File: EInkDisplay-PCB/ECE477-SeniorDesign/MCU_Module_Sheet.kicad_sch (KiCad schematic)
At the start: 20 parts, among them SW1 SW_Push_Dual_x2, U3 STM32L496ZGTxP

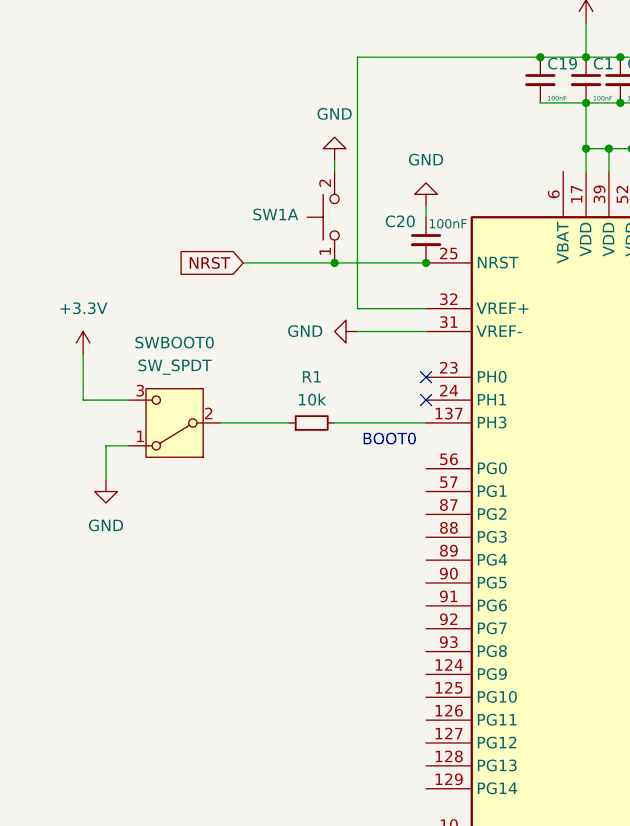
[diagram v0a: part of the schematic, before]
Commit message: Changes
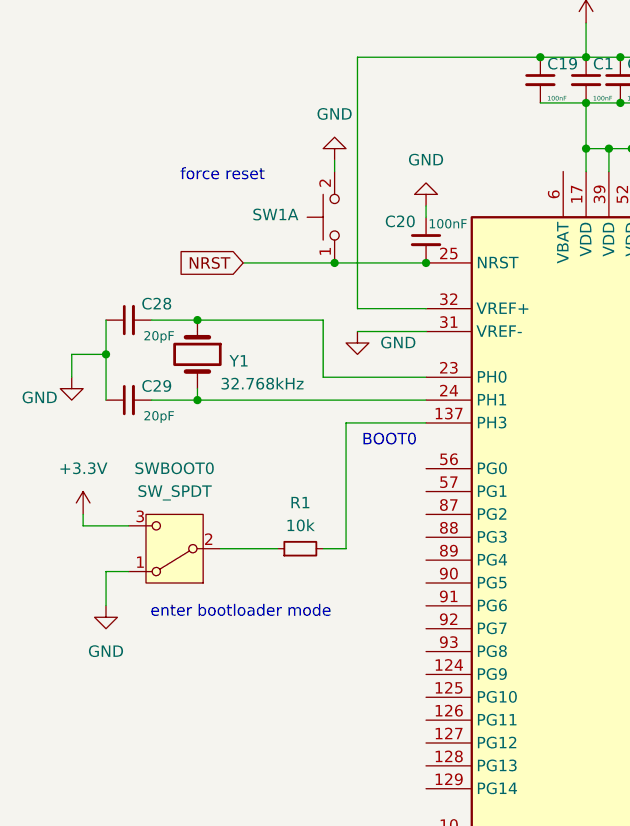
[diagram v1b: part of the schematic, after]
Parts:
- added C28, C29: 20pF, symbol Device:C_Small
- added Y1: 32.768kHz, symbol Device:Crystal
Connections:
- net GND: now also C28.1, C29.1
- net at U3.23 (PH0): now also C28.2, Y1.1
- net at U3.24 (PH1): now also C29.2, Y1.2
- no-connect marks 5 -> 3
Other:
- note added: "enter bootloader mode"
- note added: "force reset"
- moved on the sheet: R1, SWBOOT0

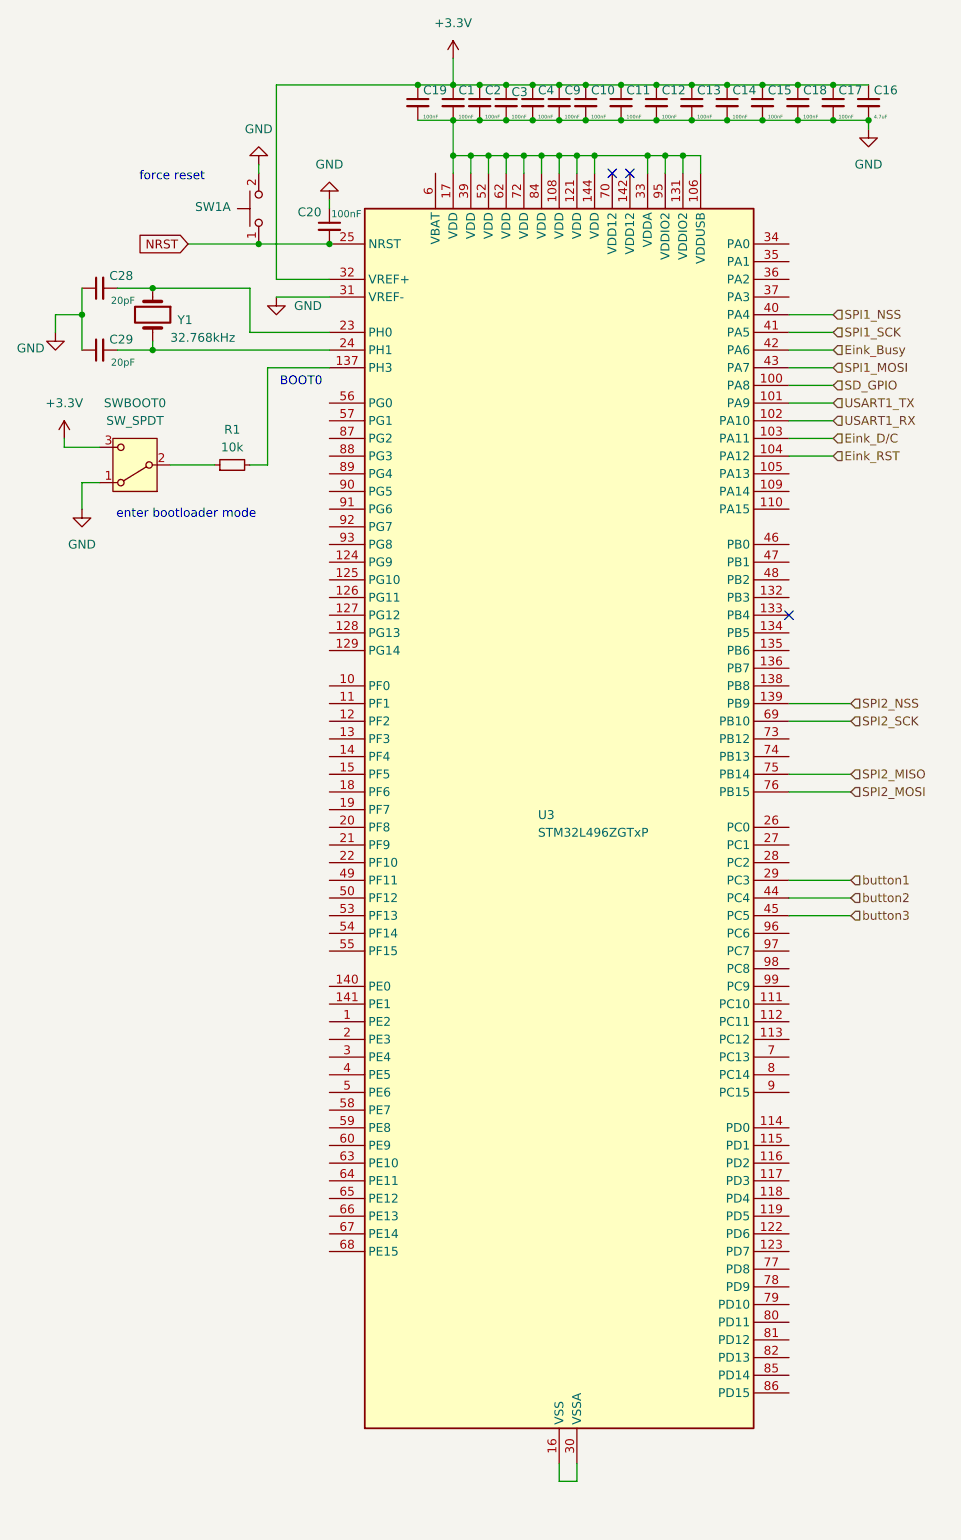
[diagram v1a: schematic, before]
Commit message: push
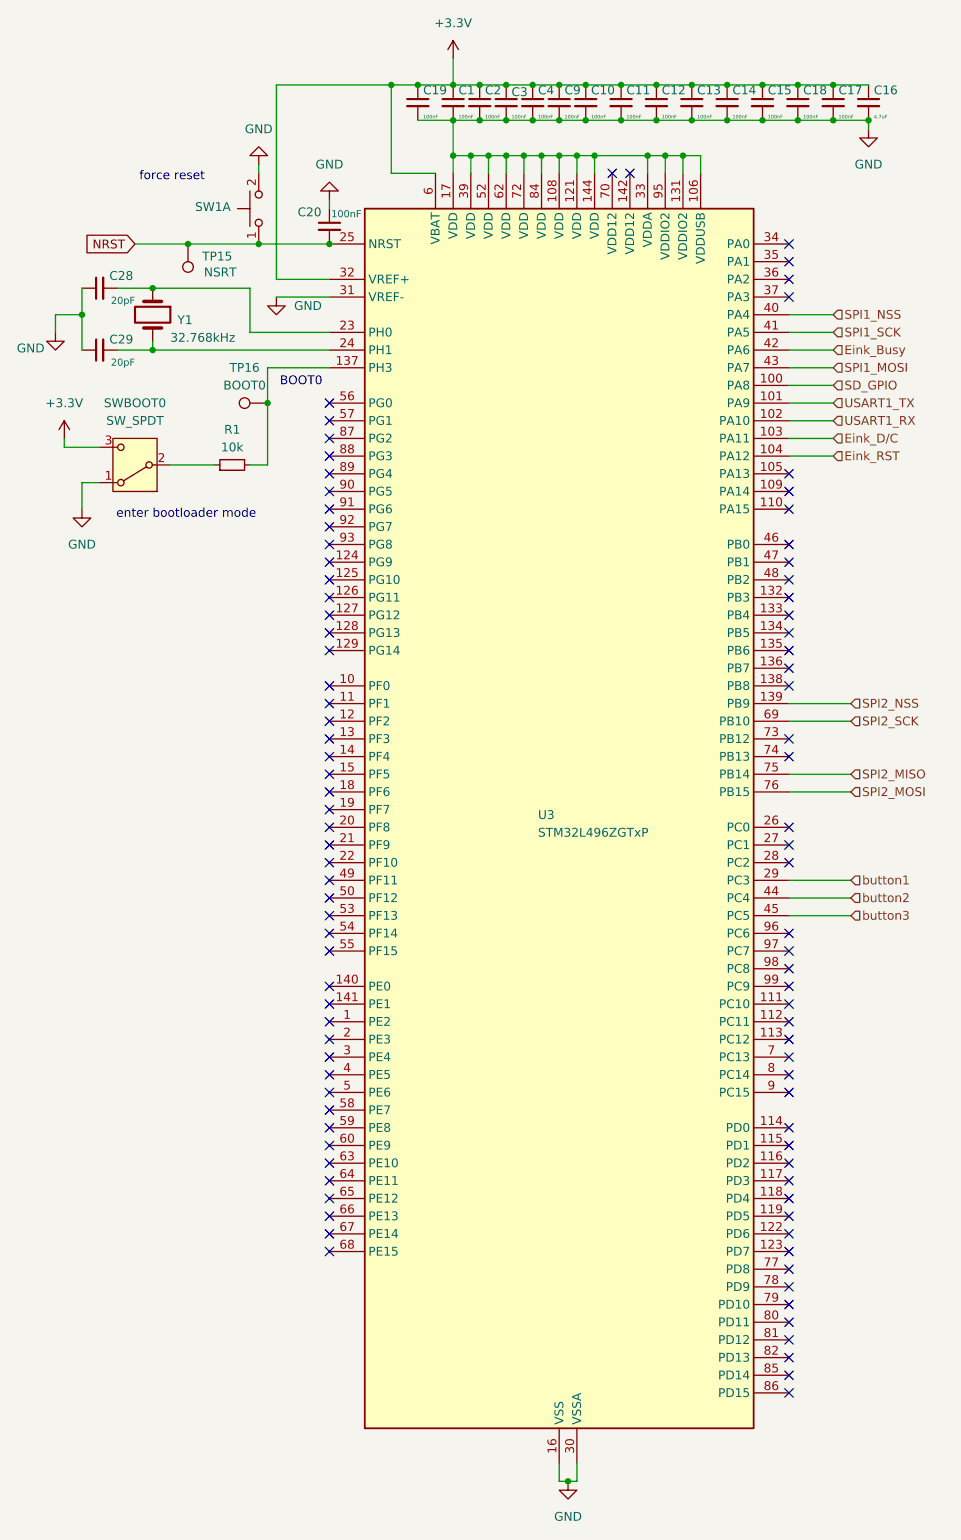
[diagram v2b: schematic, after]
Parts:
- added TP15: NSRT, symbol Connector:TestPoint
- added TP16: BOOT0, symbol Connector:TestPoint
- R1: footprint (none) -> Resistor_SMD:R_0603_1608Metric_Pad0.98x0.95mm_HandSolder
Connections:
- net +3.3V: now also U3.6 (VBAT)
- net GND: now also U3.107 (VSS), U3.120 (VSS), U3.130 (VSS), U3.143 (VSS), U3.16 (VSS), U3.30 (VSSA), U3.38 (VSS), U3.51 (VSS), U3.61 (VSS), U3.71 (VSS), U3.83 (VSS), U3.94 (VSS)
- net NRST: now also TP15.1
- net at R1.2, U3.137 (PH3): now also TP16.1
- no-connect marks 3 -> 96
